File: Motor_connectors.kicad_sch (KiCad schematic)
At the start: 3 parts

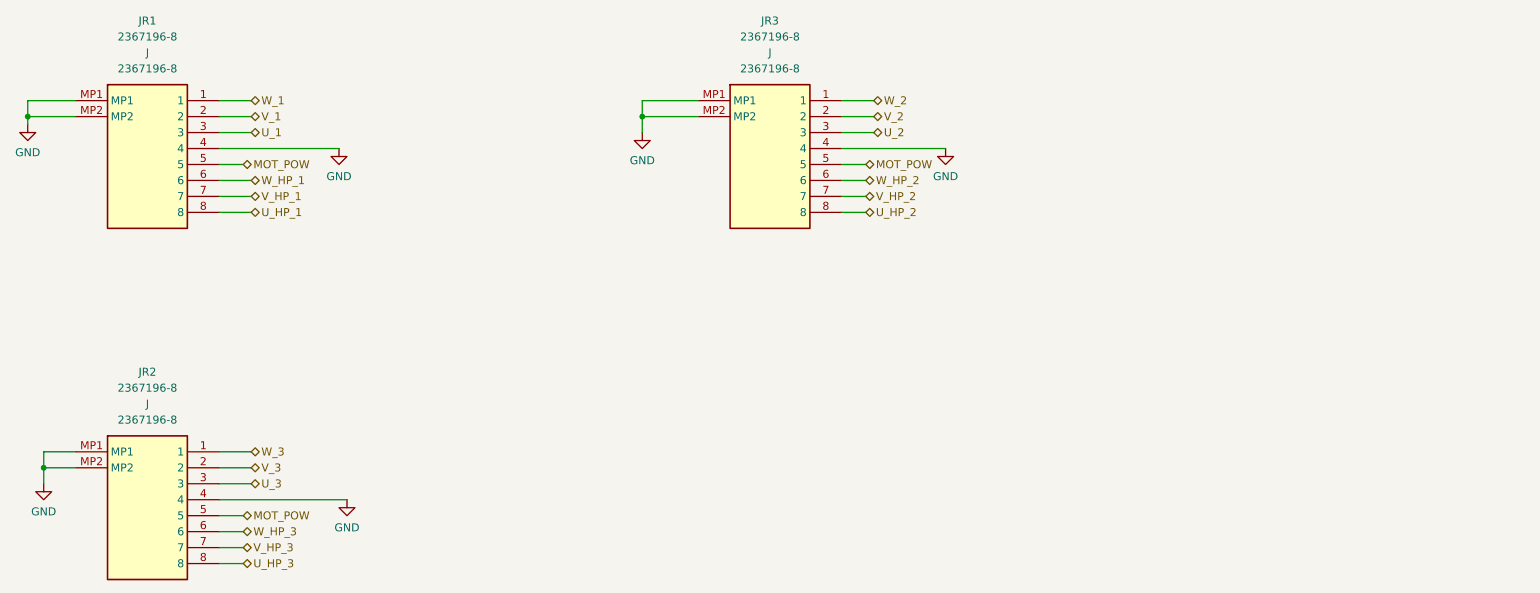
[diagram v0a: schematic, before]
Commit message: Final Schematic
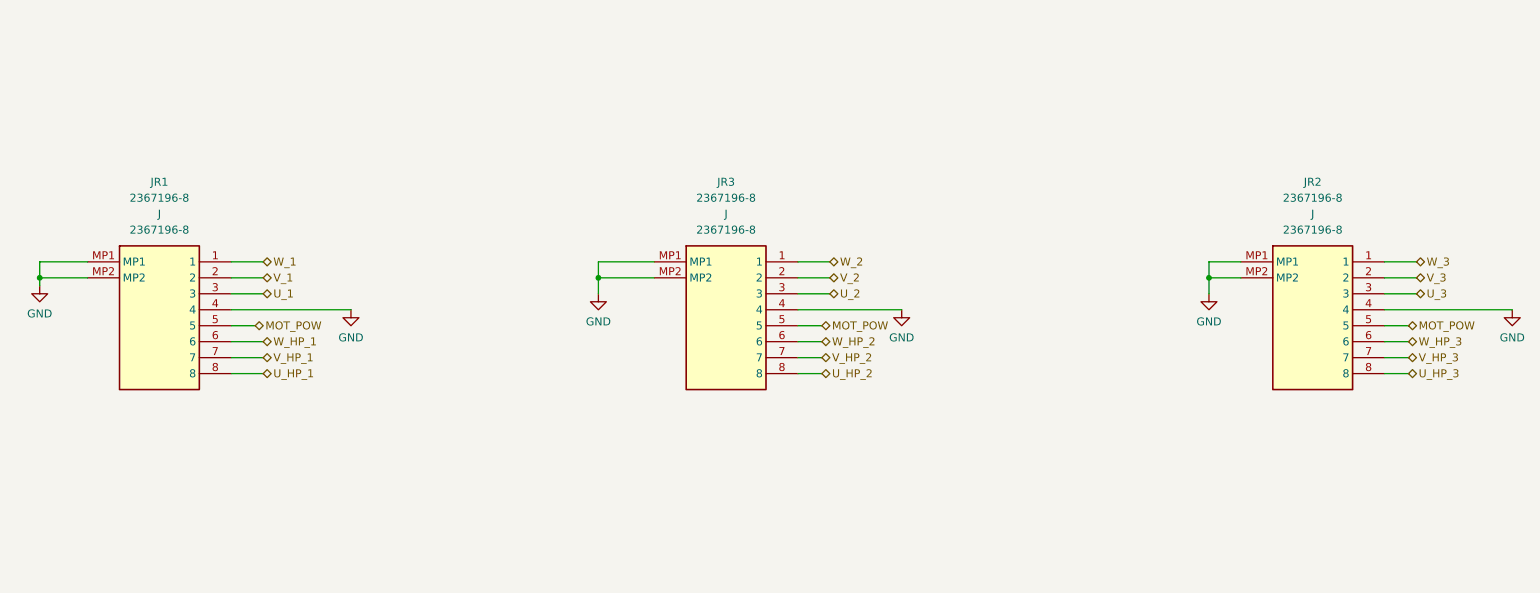
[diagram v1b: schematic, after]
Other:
- moved on the sheet: JR1, JR2, JR3
